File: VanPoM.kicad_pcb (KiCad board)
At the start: 2 copper layers, 5 parts, among them J1 Socket_ESP32-WROOM-32-NODEMCU, Q1 IPP055N03L G, Q2 IPP055N03L G, Q3 IPP120P04P4L03AKSA2, U1 BQ34Z100-R2

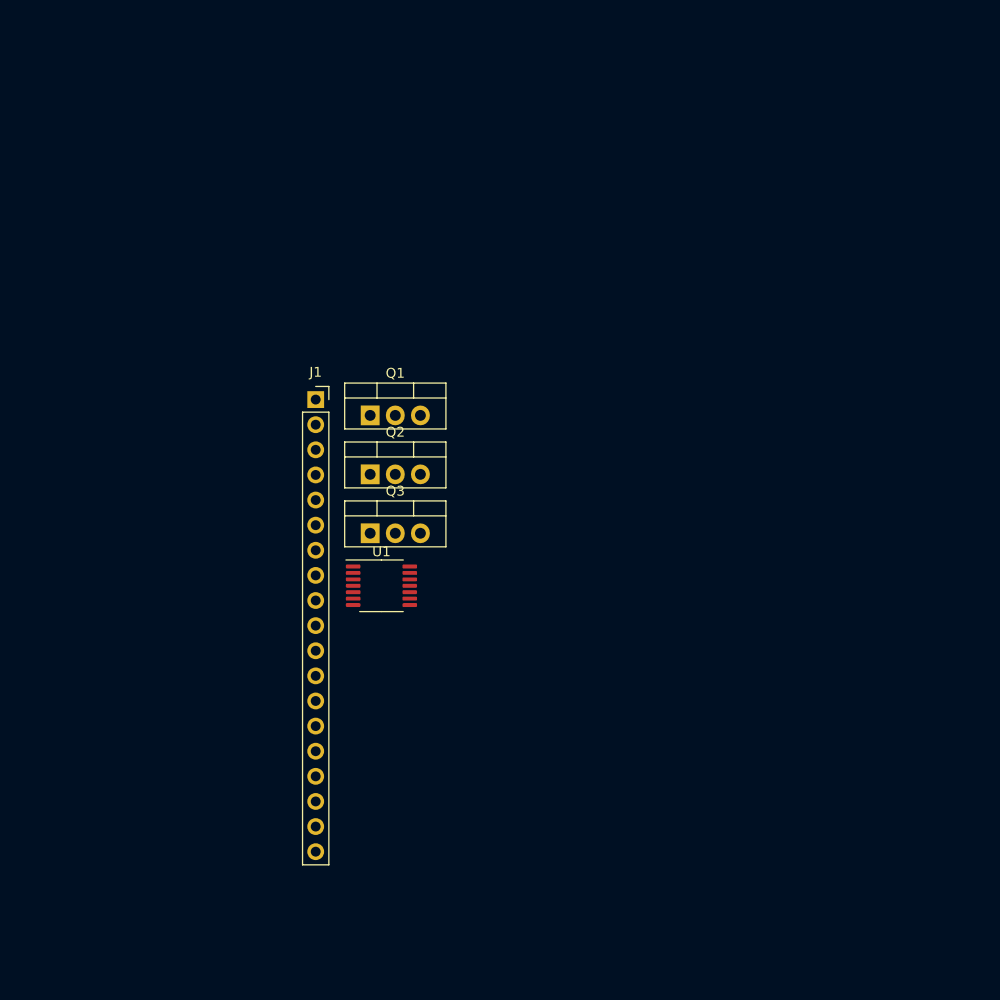
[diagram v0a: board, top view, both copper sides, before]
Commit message: +++ PCB; f many small things
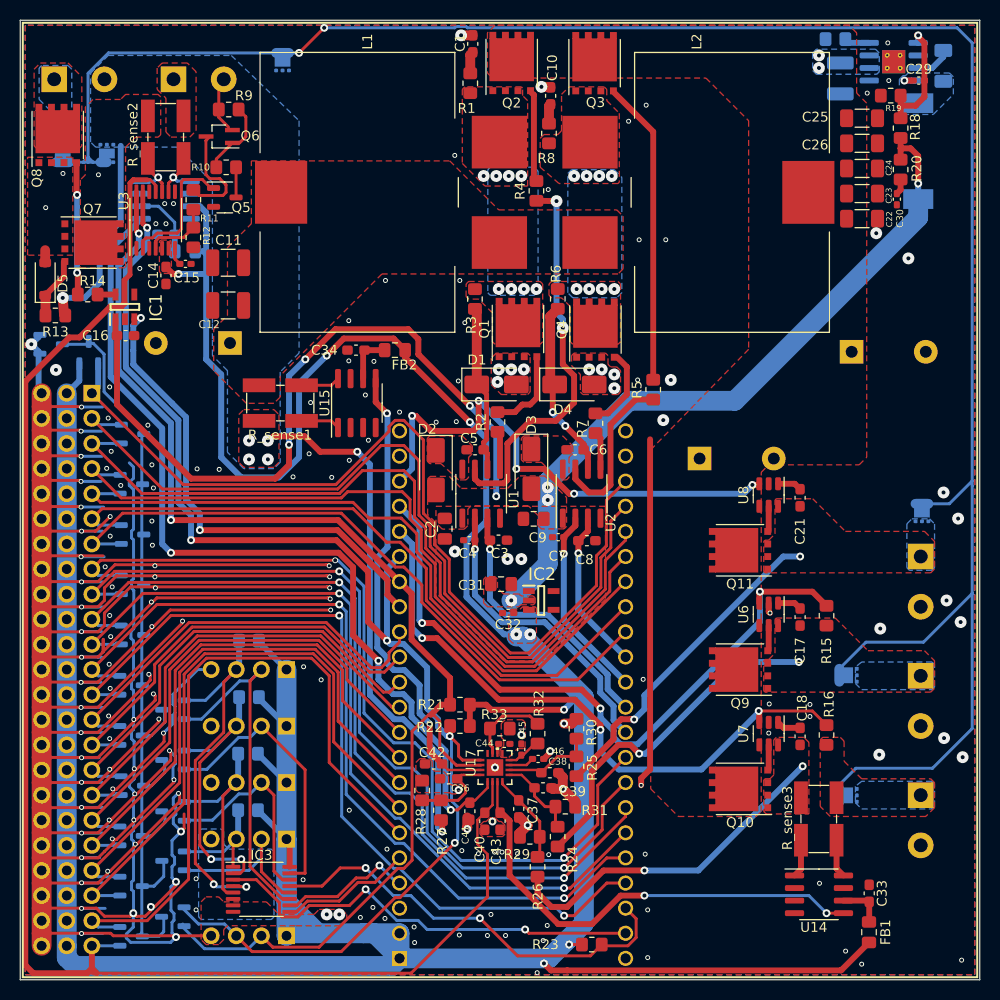
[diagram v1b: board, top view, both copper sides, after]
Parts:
- added C1: 1000p, Capacitor_SMD:C_0603_1608Metric_Pad1.08x0.95mm_HandSolder, F.Cu at (140.3, 47.8)
- added C10: 1000p, Capacitor_SMD:C_0603_1608Metric_Pad1.08x0.95mm_HandSolder, F.Cu at (148.2, 53.1)
- added C11: 10u, Capacitor_SMD:C_1210_3225Metric_Pad1.33x2.70mm_HandSolder, F.Cu at (115.6, 70.0)
- added C12: 10u, Capacitor_SMD:C_1210_3225Metric_Pad1.33x2.70mm_HandSolder, F.Cu at (115.6, 74.3)
- added C13: 1000u, Capacitor_THT:CP_Radial_D16.0mm_P7.50mm, B.Cu at (115.8, 78.1)
- added C14: 0.1u, Capacitor_SMD:C_0603_1608Metric_Pad1.08x0.95mm_HandSolder, F.Cu at (109.3, 71.3)
- added C15: 1u, Capacitor_SMD:C_0402_1005Metric_Pad0.74x0.62mm_HandSolder, F.Cu at (111.3, 70.1)
- added C16: 0.1u, Capacitor_SMD:C_0603_1608Metric_Pad1.08x0.95mm_HandSolder, F.Cu at (105.2, 77.3)
- added C17: 0.1u, Capacitor_SMD:C_0603_1608Metric_Pad1.08x0.95mm_HandSolder, F.Cu at (173.4, 105.8)
- added C18: 0.1u, Capacitor_SMD:C_0603_1608Metric_Pad1.08x0.95mm_HandSolder, F.Cu at (173.4, 117.9)
- added C19: 1200u, Capacitor_THT:CP_Radial_D18.0mm_P7.50mm, B.Cu at (163.3, 89.8)
- added C2: 1u, Capacitor_SMD:C_0805_2012Metric_Pad1.18x1.45mm_HandSolder, F.Cu at (137.5, 96.9)
- added C20: 1200u, Capacitor_THT:CP_Radial_D18.0mm_P7.50mm, B.Cu at (178.7, 79.0)
- added C21: 0.1u, Capacitor_SMD:C_0603_1608Metric_Pad1.08x0.95mm_HandSolder, F.Cu at (173.4, 93.7)
- added C22: 4.7u, Capacitor_SMD:C_1206_3216Metric_Pad1.33x1.80mm_HandSolder, F.Cu at (179.7, 65.5)
- added C23: 4.7u, Capacitor_SMD:C_1206_3216Metric_Pad1.33x1.80mm_HandSolder, F.Cu at (179.7, 63.0)
- added C24: 4.7u, Capacitor_SMD:C_1206_3216Metric_Pad1.33x1.80mm_HandSolder, F.Cu at (179.7, 60.4)
- added C25: 4.7u, Capacitor_SMD:C_1206_3216Metric_Pad1.33x1.80mm_HandSolder, F.Cu at (179.7, 55.4)
- added C26: 4.7u, Capacitor_SMD:C_1206_3216Metric_Pad1.33x1.80mm_HandSolder, F.Cu at (179.7, 57.9)
- added C27: 10u, Capacitor_SMD:C_1210_3225Metric_Pad1.33x2.70mm_HandSolder, B.Cu at (177.5, 51.3)
- added C28: 0.022u, Capacitor_SMD:C_1206_3216Metric_Pad1.33x1.80mm_HandSolder, B.Cu at (187.9, 50.1)
- added C29: 50n, Capacitor_SMD:C_0402_1005Metric_Pad0.74x0.62mm_HandSolder, F.Cu at (185.4, 51.6)
- added C3: 220p, Capacitor_SMD:C_0603_1608Metric_Pad1.08x0.95mm_HandSolder, F.Cu at (142.9, 98.0)
- added C30: 10n, Capacitor_SMD:C_0402_1005Metric_Pad0.74x0.62mm_HandSolder, F.Cu at (183.2, 63.6)
- added C31: 1u, Capacitor_SMD:C_0805_2012Metric_Pad1.18x1.45mm_HandSolder, F.Cu at (143.2, 102.5)
- added C32: 1u, Capacitor_SMD:C_0402_1005Metric_Pad0.74x0.62mm_HandSolder, F.Cu at (143.9, 105.4)
- added C33: 0.1u, Capacitor_SMD:C_0603_1608Metric_Pad1.08x0.95mm_HandSolder, F.Cu at (180.4, 133.8)
- added C34: 0.1u, Capacitor_SMD:C_0603_1608Metric_Pad1.08x0.95mm_HandSolder, F.Cu at (128.5, 78.8)
- added C35: 0.1u, Capacitor_SMD:C_0603_1608Metric_Pad1.08x0.95mm_HandSolder, B.Cu at (109.3, 67.1)
- added C36: 0.1u, Capacitor_SMD:C_0603_1608Metric_Pad1.08x0.95mm_HandSolder, F.Cu at (137.9, 122.2)
- added C37: 0.1u, Capacitor_SMD:C_0603_1608Metric_Pad1.08x0.95mm_HandSolder, F.Cu at (145.0, 125.2)
- added C38: 0.1u, Capacitor_SMD:C_0603_1608Metric_Pad1.08x0.95mm_HandSolder, F.Cu at (148.1, 121.6)
- added C39: 0.1u, Capacitor_SMD:C_0603_1608Metric_Pad1.08x0.95mm_HandSolder, F.Cu at (147.5, 123.1)
- added C4: 560p, Capacitor_SMD:C_0402_1005Metric_Pad0.74x0.62mm_HandSolder, F.Cu at (140.0, 98.0)
- added C40: 0.1u, Capacitor_SMD:C_0603_1608Metric_Pad1.08x0.95mm_HandSolder, F.Cu at (141.6, 126.5)
- added C41: 0.1u, Capacitor_SMD:C_0603_1608Metric_Pad1.08x0.95mm_HandSolder, F.Cu at (140.1, 125.4)
- added C42: 0.1u, Capacitor_SMD:C_0603_1608Metric_Pad1.08x0.95mm_HandSolder, F.Cu at (136.4, 120.7)
- added C43: 0.1u, Capacitor_SMD:C_0603_1608Metric_Pad1.08x0.95mm_HandSolder, F.Cu at (143.1, 126.5)
- added C44: 1u, Capacitor_SMD:C_0402_1005Metric_Pad0.74x0.62mm_HandSolder, F.Cu at (143.5, 118.6)
- added C45: 1u, Capacitor_SMD:C_0402_1005Metric_Pad0.74x0.62mm_HandSolder, F.Cu at (145.2, 119.2)
- added C46: 1u, Capacitor_SMD:C_0402_1005Metric_Pad0.74x0.62mm_HandSolder, F.Cu at (147.0, 120.2)
- added C5: 0.1u, Capacitor_SMD:C_0603_1608Metric_Pad1.08x0.95mm_HandSolder, F.Cu at (140.6, 88.9)
- added C6: 0.1u, Capacitor_SMD:C_0603_1608Metric_Pad1.08x0.95mm_HandSolder, F.Cu at (150.7, 88.9)
- added C7: 560p, Capacitor_SMD:C_0402_1005Metric_Pad0.74x0.62mm_HandSolder, F.Cu at (149.0, 97.7)
- added C8: 220p, Capacitor_SMD:C_0603_1608Metric_Pad1.08x0.95mm_HandSolder, F.Cu at (151.9, 98.1)
- added C9: 1u, Capacitor_SMD:C_0805_2012Metric_Pad1.18x1.45mm_HandSolder, F.Cu at (146.5, 95.9)
- added D1: B1100-13-F, Diode_SMD:D_SMA, F.Cu at (142.7, 82.3)
- added D10: PESD2USB3UXT-QR, Package_TO_SOT_SMD:SOT-23-3, B.Cu at (105.8, 133.0)
- added D11: PESD2USB3UXT-QR, Package_TO_SOT_SMD:SOT-23-3, B.Cu at (105.9, 102.5)
- added D12: PESD2USB3UXT-QR, Package_TO_SOT_SMD:SOT-23-3, B.Cu at (105.8, 127.9)
- added D13: PESD2USB3UXT-QR, Package_TO_SOT_SMD:SOT-23-3, B.Cu at (105.9, 97.5)
- added D14: PESD2USB3UXT-QR, Package_TO_SOT_SMD:SOT-23-3, B.Cu at (105.9, 122.9)
- added D15: PESD2USB3UXT-QR, Package_TO_SOT_SMD:SOT-23-3, B.Cu at (105.8, 92.4)
- added D16: PESD2USB3UXT-QR, Package_TO_SOT_SMD:SOT-23-3, B.Cu at (105.8, 117.8)
- added D17: PESD2USB3UXT-QR, Package_TO_SOT_SMD:SOT-23-3, B.Cu at (105.9, 87.3)
- added D18: PESD2USB3UXT-QR, Package_TO_SOT_SMD:SOT-23-3, B.Cu at (105.8, 112.7)
- added D2: D, Diode_SMD:D_SMA, F.Cu at (136.6, 91.0)
- added D21: PESD2USB3UXT-QR, Package_TO_SOT_SMD:SOT-23-3, B.Cu at (110.0, 115.2)
- added D22: PESD2USB3UXT-QR, Package_TO_SOT_SMD:SOT-23-3, B.Cu at (110.0, 120.3)
- added D23: PESD2USB3UXT-QR, Package_TO_SOT_SMD:SOT-23-3, B.Cu at (110.0, 125.5)
- added D24: PESD2USB3UXT-QR, Package_TO_SOT_SMD:SOT-23-3, B.Cu at (110.0, 130.5)
- added D25: PESD2USB3UXT-QR, Package_TO_SOT_SMD:SOT-23-3, B.Cu at (110.0, 136.1)
- added D3: D, Diode_SMD:D_SMA, F.Cu at (146.3, 90.8)
- added D4: B1100-13-F, Diode_SMD:D_SMA, F.Cu at (150.6, 82.3)
- added D5: BZT52C15-7-F, Diode_SMD:D_SOD-123, F.Cu at (97.1, 71.6)
- added D6: PESD2USB3UXT-QR, Package_TO_SOT_SMD:SOT-23-3, B.Cu at (97.7, 78.2)
- added D7: PESD2USB3UXT-QR, Package_TO_SOT_SMD:SOT-23-3, B.Cu at (101.5, 79.1)
- added D8: PESD2USB3UXT-QR, Package_TO_SOT_SMD:SOT-23-3, B.Cu at (105.8, 138.1)
- added D9: PESD2USB3UXT-QR, Package_TO_SOT_SMD:SOT-23-3, B.Cu at (105.9, 107.6)
- added FB1: 74279201, Capacitor_SMD:C_0805_2012Metric_Pad1.18x1.45mm_HandSolder, F.Cu at (180.4, 137.7)
- added FB2: 74279201, Capacitor_SMD:C_0805_2012Metric_Pad1.18x1.45mm_HandSolder, F.Cu at (132.5, 78.8)
- added FB3: 74279201, Capacitor_SMD:C_0805_2012Metric_Pad1.18x1.45mm_HandSolder, B.Cu at (111.2, 68.8)
- added IC1: UCC27517DBVR, Perso:SOT95P280X145-5N, F.Cu at (105.2, 74.4)
- added IC2: TLV70433DBVT, Perso:SOT95P280X145-5N, F.Cu at (147.3, 104.1)
- added IC3: SN74LV4052APWR, Package_SO:TSSOP-16_4.4x5mm_P0.65mm, F.Cu at (119.0, 133.3)
- added J10: UART1, Connector_PinHeader_2.54mm:PinHeader_1x04_P2.54mm_Vertical, B.Cu at (121.5, 128.3)
- added J11: I2C, Connector_PinHeader_2.54mm:PinHeader_1x04_P2.54mm_Vertical, B.Cu at (121.5, 138.0)
- added J2: OSTT7020150, TerminalBlock_MetzConnect:TerminalBlock_MetzConnect_Type073_RT02602HBLU_1x02_P5.08mm_Horizontal, B.Cu at (185.6, 123.8)
- added J3: OSTT7020150, TerminalBlock_MetzConnect:TerminalBlock_MetzConnect_Type073_RT02602HBLU_1x02_P5.08mm_Horizontal, B.Cu at (185.6, 99.7)
- added J4: OSTT7020150, TerminalBlock_MetzConnect:TerminalBlock_MetzConnect_Type073_RT02602HBLU_1x02_P5.08mm_Horizontal, B.Cu at (110.1, 51.4)
- added J5: OSTT7020150, TerminalBlock_MetzConnect:TerminalBlock_MetzConnect_Type073_RT02602HBLU_1x02_P5.08mm_Horizontal, B.Cu at (98.0, 51.4)
- added J6: Conn_03x23_Row_Letter_First, Perso:PinHeader_3x23_P2.54mm_Vertical, B.Cu at (101.8, 83.2)
- added J7: UART4, Connector_PinHeader_2.54mm:PinHeader_1x04_P2.54mm_Vertical, B.Cu at (121.5, 111.1)
- added J8: UART3, Connector_PinHeader_2.54mm:PinHeader_1x04_P2.54mm_Vertical, B.Cu at (121.5, 116.8)
- added J9: UART2, Connector_PinHeader_2.54mm:PinHeader_1x04_P2.54mm_Vertical, B.Cu at (121.5, 122.5)
- added L1: 22u, Inductor_SMD:L_Wuerth_HCF-2818, F.Cu at (128.7, 62.9)
- added L2: 22u, Inductor_SMD:L_Wuerth_HCF-2818, F.Cu at (166.6, 62.9)
- added L3: 220u, Perso:INDPM105103X500N, B.Cu at (185.4, 58.7)
- added Q10: CSD18540Q5B, Package_SON:VSONP-8-1EP_5x6_P1.27mm, F.Cu at (167.4, 123.2)
- added Q11: CSD18540Q5B, Package_SON:VSONP-8-1EP_5x6_P1.27mm, F.Cu at (167.4, 99.1)
- added Q4: CSD19531Q5A, Package_SON:VSONP-8-1EP_5x6_P1.27mm, F.Cu at (152.8, 76.7)
- added Q5: NX7002AK,215, Package_TO_SOT_SMD:SOT-23-3, F.Cu at (115.3, 63.4)
- added Q6: BSS84W-7-F, Package_TO_SOT_SMD:SOT-323_SC-70_Handsoldering, F.Cu at (114.7, 57.2)
- added Q7: CSD18540Q5B, Package_SON:VSONP-8-1EP_5x6_P1.27mm, F.Cu at (101.9, 67.9)
- added Q8: CSD18540Q5B, Package_SON:VSONP-8-1EP_5x6_P1.27mm, F.Cu at (98.4, 57.1)
- added Q9: CSD18540Q5B, Package_SON:VSONP-8-1EP_5x6_P1.27mm, F.Cu at (167.4, 111.1)
- added R1: 5.6, Resistor_SMD:R_0805_2012Metric_Pad1.20x1.40mm_HandSolder, F.Cu at (140.1, 51.8)
- added R10: 330k, Resistor_SMD:R_0805_2012Metric_Pad1.20x1.40mm_HandSolder, F.Cu at (115.4, 60.3)
- added R11: 390k, Resistor_SMD:R_0805_2012Metric_Pad1.20x1.40mm_HandSolder, F.Cu at (112.1, 63.6)
- added R12: 30k, Resistor_SMD:R_0805_2012Metric_Pad1.20x1.40mm_HandSolder, F.Cu at (112.1, 67.4)
- added R13: 10k, Resistor_SMD:R_0805_2012Metric_Pad1.20x1.40mm_HandSolder, F.Cu at (98.1, 75.3)
- added R14: 5.11, Resistor_SMD:R_0805_2012Metric_Pad1.20x1.40mm_HandSolder, F.Cu at (101.4, 73.2)
- added R15: 100k, Resistor_SMD:R_0805_2012Metric_Pad1.20x1.40mm_HandSolder, F.Cu at (176.1, 105.7)
- added R16: 100k, Resistor_SMD:R_0805_2012Metric_Pad1.20x1.40mm_HandSolder, F.Cu at (176.1, 117.7)
- added R17: 140k, Resistor_SMD:R_0805_2012Metric_Pad1.20x1.40mm_HandSolder, B.Cu at (177.0, 47.4)
- added R18: 220k, Resistor_SMD:R_0805_2012Metric_Pad1.20x1.40mm_HandSolder, F.Cu at (183.6, 56.4)
- added R19: 30k, Resistor_SMD:R_0805_2012Metric_Pad1.20x1.40mm_HandSolder, F.Cu at (182.6, 53.1)
- added R2: 4.42, Resistor_SMD:R_0805_2012Metric_Pad1.20x1.40mm_HandSolder, F.Cu at (142.8, 86.1)
- added R20: 3.00, Resistor_SMD:R_0805_2012Metric_Pad1.20x1.40mm_HandSolder, F.Cu at (183.6, 60.6)
- added R21: 10k, Resistor_SMD:R_0805_2012Metric_Pad1.20x1.40mm_HandSolder, F.Cu at (139.1, 114.7)
- added R22: 10k, Resistor_SMD:R_0805_2012Metric_Pad1.20x1.40mm_HandSolder, F.Cu at (139.1, 116.8)
- added R23: 100k, Resistor_SMD:R_0805_2012Metric_Pad1.20x1.40mm_HandSolder, F.Cu at (152.4, 138.9)
- added R24: 1.8M, Resistor_SMD:R_0805_2012Metric_Pad1.20x1.40mm_HandSolder, F.Cu at (148.9, 128.0)
- added R25: 1.8M, Resistor_SMD:R_0805_2012Metric_Pad1.20x1.40mm_HandSolder, F.Cu at (150.8, 120.9)
- added R26: 1.8M, Resistor_SMD:R_0805_2012Metric_Pad1.20x1.40mm_HandSolder, F.Cu at (146.9, 131.1)
- added R27: 1.8M, Resistor_SMD:R_0805_2012Metric_Pad1.20x1.40mm_HandSolder, F.Cu at (137.1, 125.4)
- added R28: 200k, Resistor_SMD:R_0805_2012Metric_Pad1.20x1.40mm_HandSolder, F.Cu at (135.2, 123.4)
- added R29: 200k, Resistor_SMD:R_0805_2012Metric_Pad1.20x1.40mm_HandSolder, F.Cu at (146.1, 128.0)
- added R3: 2.21, Resistor_SMD:R_0805_2012Metric_Pad1.20x1.40mm_HandSolder, F.Cu at (140.6, 73.7)
- added R30: 200k, Resistor_SMD:R_0805_2012Metric_Pad1.20x1.40mm_HandSolder, F.Cu at (150.8, 117.1)
- added R31: 200k, Resistor_SMD:R_0805_2012Metric_Pad1.20x1.40mm_HandSolder, F.Cu at (149.7, 125.0)
- added R32: R, Resistor_SMD:R_0805_2012Metric_Pad1.20x1.40mm_HandSolder, F.Cu at (146.9, 117.6)
- added R33: R, Resistor_SMD:R_0805_2012Metric_Pad1.20x1.40mm_HandSolder, F.Cu at (143.1, 117.1)
- added R34: 100k, Resistor_SMD:R_0805_2012Metric_Pad1.20x1.40mm_HandSolder, B.Cu at (117.6, 125.3)
- added R35: 100k, Resistor_SMD:R_0805_2012Metric_Pad1.20x1.40mm_HandSolder, B.Cu at (117.7, 113.9)
- added R36: 100k, Resistor_SMD:R_0805_2012Metric_Pad1.20x1.40mm_HandSolder, B.Cu at (117.7, 108.2)
- added R37: 100k, Resistor_SMD:R_0805_2012Metric_Pad1.20x1.40mm_HandSolder, B.Cu at (117.6, 119.6)
- added R4: 2.21, Resistor_SMD:R_0805_2012Metric_Pad1.20x1.40mm_HandSolder, F.Cu at (146.8, 62.7)
- added R5: 2.21, Resistor_SMD:R_0805_2012Metric_Pad1.20x1.40mm_HandSolder, F.Cu at (158.6, 82.8)
- added R6: 2.21, Resistor_SMD:R_0805_2012Metric_Pad1.20x1.40mm_HandSolder, F.Cu at (148.9, 73.6)
- added R7: 4.42, Resistor_SMD:R_0805_2012Metric_Pad1.20x1.40mm_HandSolder, F.Cu at (152.8, 86.2)
- added R8: 5.6, Resistor_SMD:R_0805_2012Metric_Pad1.20x1.40mm_HandSolder, F.Cu at (148.1, 56.9)
- added R9: 240k, Resistor_SMD:R_0805_2012Metric_Pad1.20x1.40mm_HandSolder, F.Cu at (115.7, 54.5)
- added R_sense1: 2m, Perso:R_Shunt_Ohmite_LVK25-fixed, F.Cu at (120.9, 84.2)
- added R_sense2: 2m, Perso:R_Shunt_Ohmite_LVK25-fixed, F.Cu at (109.3, 57.3)
- added R_sense3: 2m, Perso:R_Shunt_Ohmite_LVK25-fixed, F.Cu at (175.3, 126.2)
- added U10: LM5163DDAR, Perso:SOIC-8-1EP_3.9x4.9mm_P1.27mm_EP2.34x2.34mm_ThermalVias, B.Cu at (182.9, 49.7)
- added U11: TVS3300DRV, Package_SON:WSON-6-1EP_2x2mm_P0.65mm_EP1x1.6mm, B.Cu at (103.3, 58.9)
- added U12: TVS3300DRV, Package_SON:WSON-6-1EP_2x2mm_P0.65mm_EP1x1.6mm, B.Cu at (121.1, 49.7)
- added U13: ESP32-S3-DEVKITC-1-N16R2, Perso:XCVR_ESP32-S3-DEVKITC-1, B.Cu at (144.4, 110.4)
- added U14: INA240A2D, Package_SO:SOIC-8_3.9x4.9mm_P1.27mm, F.Cu at (175.4, 133.9)
- added U15: INA240A2D, Package_SO:SOIC-8_3.9x4.9mm_P1.27mm, F.Cu at (128.6, 84.2)
- added U16: INA240A2D, Package_SO:SOIC-8_3.9x4.9mm_P1.27mm, B.Cu at (109.3, 63.6)
- added U17: TLA2528IRTER, Perso:WQFN16_RTE_TEX-L, F.Cu at (142.6, 121.0)
- added U18: TVS3300DRV, Package_SON:WSON-6-1EP_2x2mm_P0.65mm_EP1x1.6mm, B.Cu at (98.9, 58.9)
- added U2: LM5109BMA/NOPB, Package_SO:SOIC-8_3.9x4.9mm_P1.27mm, F.Cu at (151.4, 93.3)
- added U3: BQ34Z100-R2, Package_SO:TSSOP-14_4.4x5mm_P0.65mm, F.Cu at (108.3, 65.7)
- added U4: TVS3300DRV, Package_SON:WSON-6-1EP_2x2mm_P0.65mm_EP1x1.6mm, B.Cu at (178.3, 111.7)
- added U5: TVS3300DRV, Package_SON:WSON-6-1EP_2x2mm_P0.65mm_EP1x1.6mm, B.Cu at (178.3, 123.8)
- added U6: LM74700, Package_TO_SOT_SMD:SOT-23-6, F.Cu at (170.3, 105.5)
- added U7: LM74700, Package_TO_SOT_SMD:SOT-23-6, F.Cu at (170.3, 117.6)
- added U8: LM74700, Package_TO_SOT_SMD:SOT-23-6, F.Cu at (170.3, 93.5)
- added U9: TVS3300DRV, Package_SON:WSON-6-1EP_2x2mm_P0.65mm_EP1x1.6mm, B.Cu at (185.8, 95.2)
- J1: value Socket_ESP32-WROOM-32-NODEMCU -> OSTT7020150; footprint Connector_PinSocket_2.54mm:PinSocket_1x19_P2.54mm_Vertical -> TerminalBlock_MetzConnect:TerminalBlock_MetzConnect_Type073_RT02602HBLU_1x02_P5.08mm_Horizontal; moved to B.Cu
- Q1, Q2: value IPP055N03L G -> CSD19531Q5A; footprint Package_TO_SOT_THT:TO-220-3_Vertical -> Package_SON:VSONP-8-1EP_5x6_P1.27mm
- Q3: value IPP120P04P4L03AKSA2 -> CSD19531Q5A; footprint Package_TO_SOT_THT:TO-220-3_Vertical -> Package_SON:VSONP-8-1EP_5x6_P1.27mm
- U1: value BQ34Z100-R2 -> LM5109BMA/NOPB; footprint Package_SO:TSSOP-14_4.4x5mm_P0.65mm -> Package_SO:SOIC-8_3.9x4.9mm_P1.27mm
- moved J1 67.3 mm to (185.6, 111.8), turned to -90 degrees
- moved Q3 52.7 mm to (152.7, 49.8), turned to 90 degrees
- moved Q2 44.0 mm to (144.3, 49.8), turned to 90 degrees
- moved Q1 17.3 mm to (144.9, 76.7), turned to 90 degrees
- moved U1 13.7 mm to (141.2, 93.3), turned to 90 degrees
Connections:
- J1 pad 1: unconnected-(J1-5V-Pad1) -> V_S
- J1 pad 2: unconnected-(J1-CLK-Pad2) -> P-
- Q1 pad 1: Net-(D1-K) -> P-
- Q1 pad 2: BAT + -> Net-(Q1-S-Pad2)
- Q1 pad 3: (no net) -> Net-(L1-Pad2)
- Q2 pad 1: BAT - -> Net-(L1-Pad2)
- Q2 pad 3: (no net) -> V_IN
- Q3 pad 3: BAT + -> V_IN
- U1 pad 1: BAT - -> +10V
- U1 pad 2: Net-(Q2-G) -> PW_H1
- U1 pad 3: BAT - -> PW_L1
- U1 pad 4: Net-(U1-BAT) -> P-
- U1 pad 5: Net-(Q1-3) -> Net-(U1-LO)
- U1 pad 6: Net-(Q1-3) -> Net-(D1-K)
- U1 pad 7: unconnected-(U1-REG25-Pad7) -> Net-(U1-HO)
- U1 pad 8: BAT - -> Net-(D2-K)
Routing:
- net P-: track 0.00 -> 606.7 mm, vias 0 -> 189
- net +3V3: track 0.00 -> 372.3 mm, vias 0 -> 8
- net TVS: track 0.00 -> 222.3 mm, vias 0 -> 2
- net 103AT: track 0.00 -> 158.9 mm
- net +10V: track 0.00 -> 146.1 mm, vias 0 -> 8
- net SCL: track 0.00 -> 139.4 mm, vias 0 -> 5
- net SDA: track 0.00 -> 132.7 mm, vias 0 -> 2
- net GPIO19: track 0.00 -> 93.1 mm
- net AIO_2: track 0.00 -> 91.1 mm, vias 0 -> 3
- net GPIO39: track 0.00 -> 88.7 mm, vias 0 -> 2
- net GPIO20: track 0.00 -> 87.1 mm
- net GPIO40: track 0.00 -> 86.8 mm, vias 0 -> 2
- net TVS_3v3: track 0.00 -> 86.3 mm
- net GPIO1: track 0.00 -> 86.2 mm, vias 0 -> 2
- net GPIO41: track 0.00 -> 85.7 mm, vias 0 -> 2
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- added copper zone on F.Cu, net +10V
- added copper zone on F.Cu, net +3V3
- added copper zone on B.Cu, net BAT+
- added copper zone on F.Cu, net BAT+
- added copper zone on F.Cu, net BAT-
- added copper zone on F.Cu, net Net-(C11-Pad1)
- added copper zone on F.Cu, net Net-(D2-K)
- added copper zone on F.Cu, net Net-(D3-K)
- added copper zone on B.Cu, net Net-(L1-Pad2)
- added copper zone on F.Cu, net Net-(L1-Pad2)
- added copper zone on B.Cu, net Net-(L2-Pad1)
- added copper zone on F.Cu, net Net-(L2-Pad1)
- added copper zone on F.Cu, net Net-(Q7-S-Pad3)
- added copper zone on B.Cu, net Net-(U10-SW)
- added copper zone on B.Cu, net OUT-
- added copper zone on F.Cu, net OUT-
- added copper zone on B.Cu, net P+
- added copper zone on F.Cu, net P+
- added copper zone on B.Cu, net P-
- added copper zone on F.Cu, net P-
- added copper zone on B.Cu, net V_A
- added copper zone on F.Cu, net V_A
- added copper zone on B.Cu, net V_IN
- added copper zone on F.Cu, net V_IN
- added copper zone on F.Cu, net V_P
- added copper zone on B.Cu, net V_S
- added copper zone on F.Cu, net V_S
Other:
- board outline added: 97 x 97 mm
- board text added: "+"
- board text added: "+15V INPUT (FROM AC/DC CONVERTER)"
- board text added: "00"
- board text added: "01"
- board text added: "02"
- board text added: "03"
- board text added: "06"
- board text added: "07"
- board text added: "08"
- board text added: "15"
- board text added: "16"
- board text added: "17"
- board text added: "18"
- board text added: "19"
- board text added: "20"
- board text added: "21"
- board text added: "39"
- board text added: "3V3"
- board text added: "40"
- board text added: "41"
- board text added: "42"
- board text added: "45"
- board text added: "46"
- board text added: "47"
- board text added: "48"
- board text added: "BAT TEMP"
- board text added: "BATTERY"
- board text added: "CAR BATTERY"
- board text added: "GND"
- board text added: "I2C"
- board text added: "IO"
- board text added: "LOAD"
- board text added: "RX"
- board text added: "SCL"
- board text added: "SDA"
- board text added: "SOLAR PANELS"
- board text added: "TX"
- board text added: "UART1"
- board text added: "UART2"
- board text added: "UART3"
- board text added: "UART4"
- board text added: "VanPom v1.0 Copyright © Léo Flaventin Hauchecorne https://github.com/hl037/VanPom"
- board text added: "−"
